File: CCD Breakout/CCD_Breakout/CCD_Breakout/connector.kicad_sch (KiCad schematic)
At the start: 3 parts

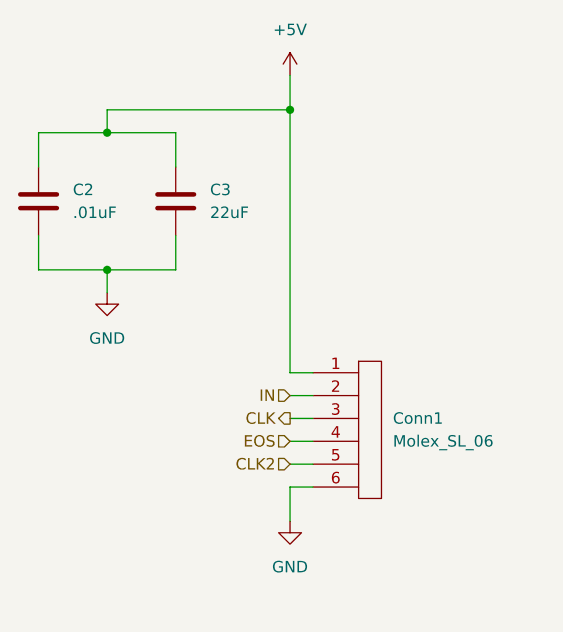
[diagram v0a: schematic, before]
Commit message: ST and EOS Pin Connections
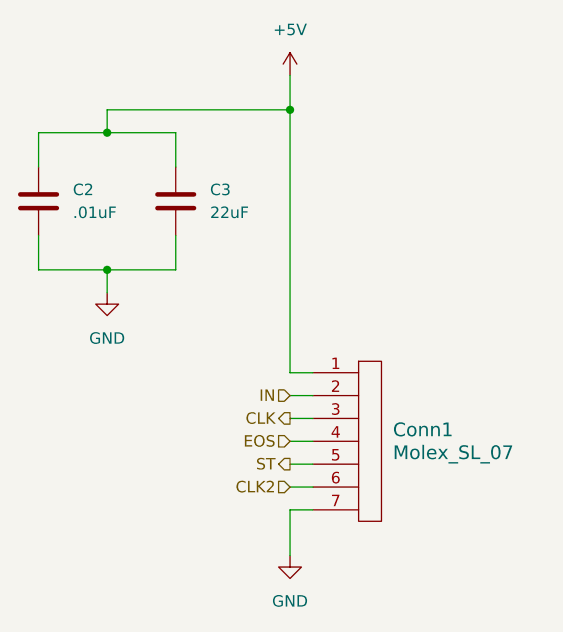
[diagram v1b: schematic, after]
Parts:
- removed Conn1: Molex_SL_06, symbol MRDT_Connectors:Molex_SL_06
- added Conn1: Molex_SL_07, symbol MRDT_Connectors:Molex_SL_07
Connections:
- net +5V: now also Conn1.1
- net CLK: now also Conn1.3
- net CLK2: now also Conn1.6
- net EOS: now also Conn1.4
- net GND: now also Conn1.7
- net IN: now also Conn1.2
- new net ST: Conn1.5
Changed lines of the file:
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@@
+	(wire
+		(pts
+			(xy 152.4 110.49) (xy 149.86 110.49)
+		)
+		(stroke
+			(width 0)
+			(type default)
+		)
+	)
 	(wire
 		(pts
@@
 	(wire
 		(pts
+			(xy 149.86 110.49) (xy 149.86 115.57)
+		)
+		(stroke
+			(width 0)
+			(type default)
+		)
+	)
+	(wire
+		(pts
+			(xy 149.86 102.87) (xy 152.4 102.87)
+		)
+		(stroke
+			(width 0)
+			(type default)
+		)
+	)
+	(wire
+		(pts
+			(xy 149.86 62.23) (xy 149.86 66.04)
+		)
+		(stroke
+			(width 0)
+			(type default)
+		)
+	)
+	(wire
+		(pts
+			(xy 129.54 66.04) (xy 149.86 66.04)
+		)
+		(stroke
+			(width 0)
+			(type default)
+		)
+	)
+	(wire
+		(pts
+			(xy 152.4 95.25) (xy 149.86 95.25)
+		)
+		(stroke
+			(width 0)
+			(type default)
+		)
+	)
+	(wire
+		(pts
+			(xy 121.92 83.82) (xy 129.54 83.82)
+		)
+		(stroke
+			(width 0)
+			(type default)
+		)
+	)
+	(wire
+		(pts
+			(xy 149.86 107.95) (xy 152.4 107.95)
+		)
+		(stroke
+			(width 0)
+			(type default)
+		)
+	)
+	(wire
+		(pts
+			(xy 149.86 100.33) (xy 152.4 100.33)
+		)
+		(stroke
+			(width 0)
+			(type default)
+		)
+	)
+	(wire
+		(pts
+			(xy 121.92 80.01) (xy 121.92 83.82)
+		)
+		(stroke
+			(width 0)
+			(type default)
+		)
+	)
+	(wire
+		(pts
+			(xy 137.16 80.01) (xy 137.16 83.82)
+		)
+		(stroke
+			(width 0)
+			(type default)
+		)
+	)
+	(wire
+		(pts
 			(xy 149.86 105.41) (xy 152.4 105.41)
-		)
-		(stroke
-			(width 0)
-			(type default)
-		)
-	)
-	(wire
-		(pts
-			(xy 149.86 111.76) (xy 149.86 107.95)
-		)
-		(stroke
-			(width 0)
-			(type default)
-		)
-	)
-	(wire
-		(pts
-			(xy 149.86 102.87) (xy 152.4 102.87)
-		)
-		(stroke
-			(width 0)
-			(type default)
-		)
-	)
-	(wire
-		(pts
-			(xy 149.86 62.23) (xy 149.86 66.04)
-		)
-		(stroke
-			(width 0)
-			(type default)
-		)
-	)
-	(wire
-		(pts
-			(xy 129.54 66.04) (xy 149.86 66.04)
-		)
-		(stroke
-			(width 0)
-			(type default)
-		)
-	)
-	(wire
-		(pts
-			(xy 149.86 107.95) (xy 152.4 107.95)
-		)
-		(stroke
-			(width 0)
-			(type default)
-		)
-	)
-	(wire
-		(pts
-			(xy 152.4 95.25) (xy 149.86 95.25)
-		)
-		(stroke
-			(width 0)
-			(type default)
-		)
-	)
-	(wire
-		(pts
-			(xy 121.92 83.82) (xy 129.54 83.82)
-		)
-		(stroke
-			(width 0)
-			(type default)
-		)
-	)
-	(wire
-		(pts
-			(xy 149.86 100.33) (xy 152.4 100.33)
-		)
-		(stroke
-			(width 0)
-			(type default)
-		)
-	)
-	(wire
-		(pts
-			(xy 121.92 80.01) (xy 121.92 83.82)
-		)
-		(stroke
-			(width 0)
-			(type default)
-		)
-	)
-	(wire
-		(pts
-			(xy 137.16 80.01) (xy 137.16 83.82)
 		)
 		(stroke
@@
 		)
 	)
+	(hierarchical_label "ST"
+		(shape output)
+		(at 149.86 105.41 180)
+		(effects
+			(font
+				(size 1.27 1.27)
+			)
+			(justify right)
+		)
+	)
 	(hierarchical_label "EOS"
 		(shape input)
@@
 	(hierarchical_label "CLK2"
 		(shape input)
-		(at 149.86 105.41 180)
+		(at 149.86 107.95 180)
 		(effects
 			(font
@@
 	(symbol
 		(lib_id "power:GND")
-		(at 149.86 111.76 0)
+		(at 149.86 115.57 0)
 		(unit 1)
 		(exclude_from_sim no)
@@
 		(fields_autoplaced yes)
 		(property "Reference" "#PWR09"
-			(at 149.86 118.11 0)
+			(at 149.86 121.92 0)
 			(effects
 				(font
@@
 		)
 		(property "Value" "GND"
-			(at 149.86 116.84 0)
+			(at 149.86 120.65 0)
 			(effects
 				(font
@@
 		)
 		(property "Footprint" ""
-			(at 149.86 111.76 0)
+			(at 149.86 115.57 0)
 			(effects
 				(font
@@
 		)
 		(property "Datasheet" ""
-			(at 149.86 111.76 0)
+			(at 149.86 115.57 0)
 			(effects
 				(font
@@
 		)
 		(property "Description" "Power symbol creates a global label with name \"GND\" , ground"
-			(at 149.86 111.76 0)
+			(at 149.86 115.57 0)
 			(effects
 				(font
@@
 	)
 	(symbol
-		(lib_id "MRDT_Connectors:Molex_SL_06")
-		(at 157.48 109.22 0)
-		(unit 1)
-		(exclude_from_sim no)
-		(in_bom yes)
-		(on_board yes)
-		(dnp no)
-		(fields_autoplaced yes)
-		(property "Reference" "Conn1"
-			(at 161.29 100.3299 0)
-			(effects
-				(font
-					(size 1.27 1.27)
-				)
-				(justify left)
-			)
-		)
-		(property "Value" "Molex_SL_06"
-			(at 161.29 102.8699 0)
-			(effects
-				(font
-					(size 1.27 1.27)
-				)
-				(justify left)
-			)
-		)
-		(property "Footprint" ""
-			(at 152.4 105.41 0)
-			(effects
-				(font
-					(size 1.27 1.27)
-				)
-				(hide yes)
-			)
-		)
-		(property "Datasheet" ""
-			(at 152.4 105.41 0)
-			(effects
-				(font
-					(size 1.27 1.27)
-				)
-				(hide yes)
-			)
-		)
-		(property "Description" ""
-			(at 152.4 105.41 0)
-			(effects
-				(font
-					(size 1.27 1.27)
-				)
-				(hide yes)
-			)
-		)
-		(pin "1"
-		)
-		(pin "3"
-		)
-		(pin "5"
-		)
-		(pin "2"
-		)
-		(pin "4"
-		)
-		(pin "6"
-		)
-		(instances
-			(project ""
-				(path "/102965ac-29c6-4f96-94a4-d07431f6d693/dbede1ef-0855-4322-ae3b-1b9092ecc0c1"
-					(reference "Conn1")
-					(unit 1)
-				)
-			)
-		)
-	)
-	(symbol
 		(lib_id "power:GND")
 		(at 129.54 86.36 0)
@@
 					(unit 1)
 				)
+			)
+		)
+	)
+	(symbol
+		(lib_id "MRDT_Connectors:Molex_SL_07")
+		(at 157.48 111.76 0)
+		(unit 1)
+		(exclude_from_sim no)
+		(in_bom yes)
+		(on_board yes)
+		(dnp no)
+		(fields_autoplaced yes)
+		(property "Reference" "Conn1"
+			(at 161.29 101.5999 0)
+			(effects
+				(font
+					(size 1.524 1.524)
+				)
+				(justify left)
+			)
+		)
+		(property "Value" "Molex_SL_07"
+			(at 161.29 104.1399 0)
+			(effects
+				(font
+					(size 1.524 1.524)
+				)
+				(justify left)
+			)
+		)
+		(property "Footprint" ""
+			(at 157.48 106.68 0)
+			(effects
+				(font
+					(size 1.524 1.524)
+				)
+				(hide yes)
+			)
+		)
+		(property "Datasheet" ""
+			(at 157.48 106.68 0)
+			(effects
+				(font
+					(size 1.524 1.524)
+				)
+				(hide yes)
+			)
+		)
+		(property "Description" ""
+			(at 157.48 111.76 0)
+			(effects
+				(font
+					(size 1.27 1.27)
+				)
+				(hide yes)
+			)
+		)
+		(pin "5"
+		)
+		(pin "1"
+		)
+		(pin "3"
+		)
+		(pin "2"
+		)
+		(pin "4"
+		)
+		(pin "6"
+		)
+		(pin "7"
+		)
+		(instances
+			(project ""
+				(path "/102965ac-29c6-4f96-94a4-d07431f6d693/dbede1ef-0855-4322-ae3b-1b9092ecc0c1"
+					(reference "Conn1")
+					(unit 1)
+				)

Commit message: Fixed CCD Footprints
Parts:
- C2, C3: footprint (none) -> Capacitor_SMD:C_0603_1608Metric_Pad1.08x0.95mm_HandSolder
- Conn1: footprint (none) -> MRDT_Connectors:MOLEX_SL_07_Vertical
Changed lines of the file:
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@@
 			)
 		)
-		(property "Footprint" ""
+		(property "Footprint" "Capacitor_SMD:C_0603_1608Metric_Pad1.08x0.95mm_HandSolder"
 			(at 138.1252 80.01 0)
 			(effects
@@
 			)
 		)
-		(property "Footprint" ""
+		(property "Footprint" "MRDT_Connectors:MOLEX_SL_07_Vertical"
 			(at 157.48 106.68 0)
 			(effects
@@
 			)
 		)
-		(property "Footprint" ""
+		(property "Footprint" "Capacitor_SMD:C_0603_1608Metric_Pad1.08x0.95mm_HandSolder"
 			(at 122.8852 80.01 0)
 			(effects
